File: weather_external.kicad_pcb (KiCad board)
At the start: 2 copper layers, 33.2 x 36.1 mm, 13 parts, among them J1 Conn_01x02_Male, J2 Conn_01x02_Male, SW1 SW_Push

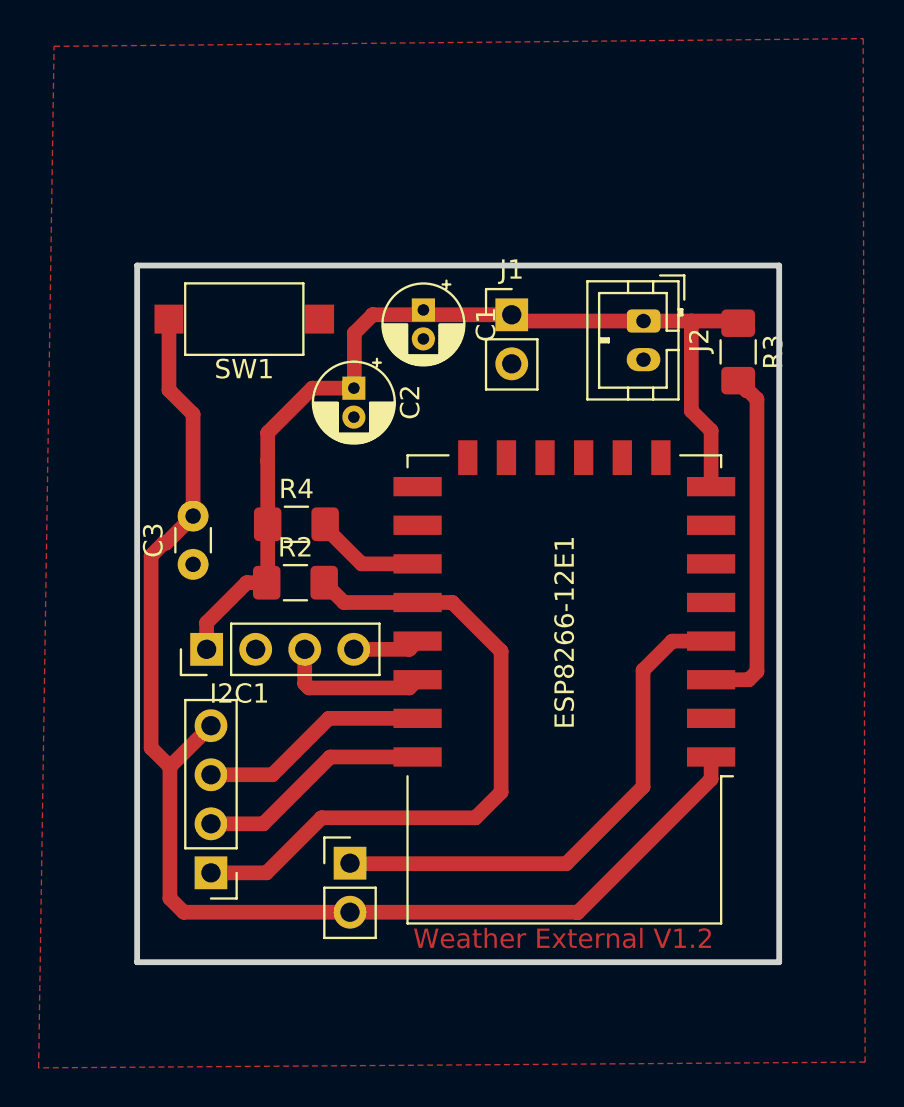
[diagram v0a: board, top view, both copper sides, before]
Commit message: JLCPCB version 1.3
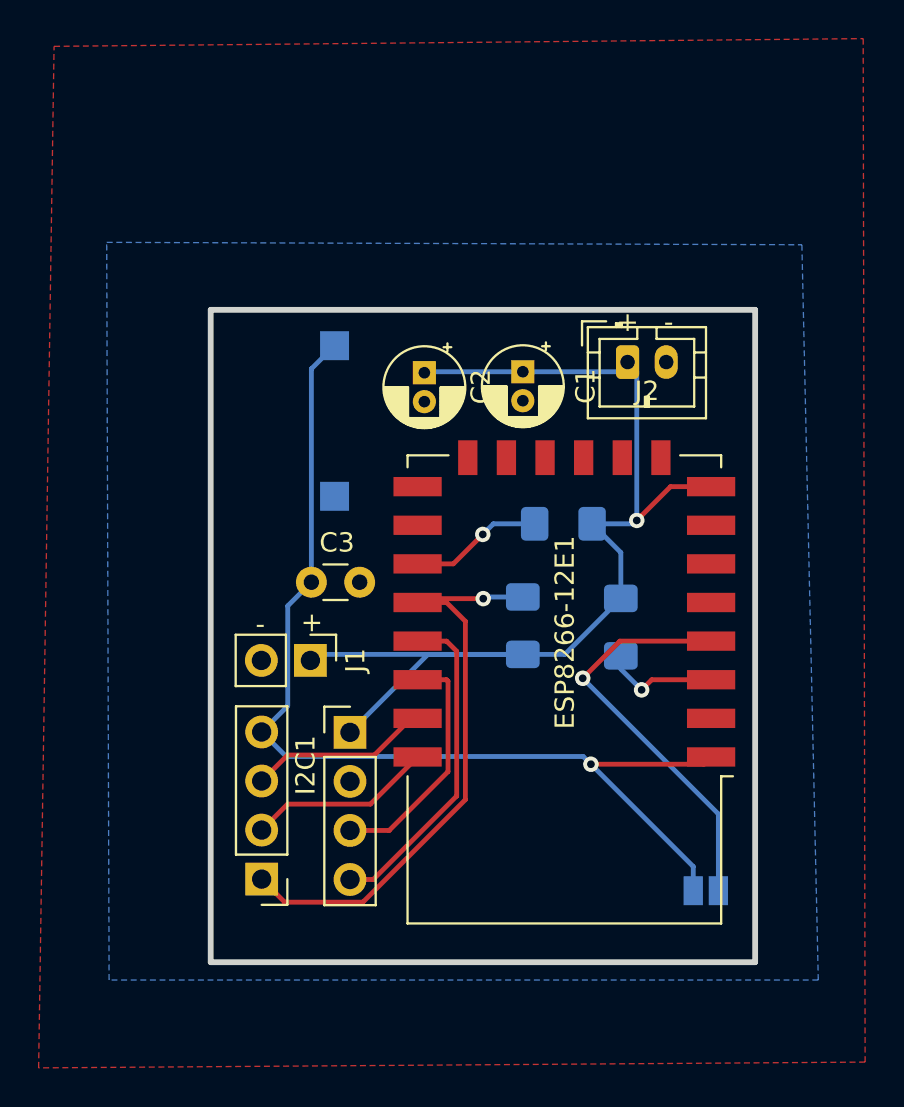
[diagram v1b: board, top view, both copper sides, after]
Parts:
- JP1: footprint Connector_PinHeader_2.54mm:PinHeader_1x02_P2.54mm_Vertical -> Jumper:SolderJumper-2_P1.3mm_Open_Pad1.0x1.5mm; moved to B.Cu
- R2, R3, R4, SW1: moved to B.Cu
- moved J1 20.7 mm to (1.10, 82.9), turned to 270 degrees
- moved JP1 18.5 mm to (21.6, 94.8), turned to 180 degrees
- moved R3 15.5 mm to (17.2, 81.2)
- moved R4 13.8 mm to (14.2, 75.8), turned to 180 degrees
- moved R2 12.0 mm to (12.1, 81.1), turned to 90 degrees
- moved C3 8.67 mm to (3.65, 78.9), turned to 180 degrees
- moved I2C1 8.58 mm to (3.15, 86.7), turned to 0 degrees
- moved SW1 7.05 mm to (2.35, 70.5), turned to 90 degrees
- moved C1 6.06 mm to (12.1, 68.0)
- moved C2 3.74 mm to (7.00, 68.0)
- moved FTDI1 2.65 mm to (-1.43, 94.2)
- moved J2 2.28 mm to (17.5, 67.5), turned to 0 degrees
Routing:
- net SDA: track 3.48 -> 17.1 mm
- net RST: track 67.2 -> 54.6 mm, vias 0 -> 1
- net EN: track 18.1 -> 6.03 mm, vias 0 -> 1
- net +3V3: track 51.0 -> 58.6 mm, vias 0 -> 1
- net GPIO16: track 27.0 -> 21.4 mm, vias 0 -> 1
- net SCL: track 7.89 -> 12.6 mm
- net GPIO0: track 34.7 -> 30.9 mm, vias 0 -> 1
- net RX: track 12.1 -> 9.42 mm
- net TX: track 12.1 -> 9.64 mm
- net GPIO2: track 5.73 -> 6.92 mm, vias 0 -> 1
- added copper zone on B.Cu, net GPIO15
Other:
- board size 33.2 x 36.1 mm -> 28.2 x 33.8 mm
- board text added: "+"
- board text added: "-"
- board text added: "EN/DIS deepsleep"
- board text added: "IO0"
- board text added: "RST"
- board text added: "RX"
- board text added: "SCL"
- board text added: "SDA"
- board text added: "TX"
- board text added: "Weather External v1.3"
- board text removed: "Weather External V1.2"
